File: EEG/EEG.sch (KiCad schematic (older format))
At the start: 1 part

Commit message: ...
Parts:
- gave numbers to parts that had none: 1
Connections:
- net labels added: +5V, GND
- wire segments 0 -> 3
- no-connect marks 0 -> 2
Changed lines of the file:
@@
 $EndDescr
 $Comp
-L Connector:USB_B_Micro J?
+L Connector:USB_B_Micro J1
 U 1 1 603925D3
 P 1950 2800
-F 0 "J?" H 2007 3267 50  0000 C CNN
+F 0 "J1" H 2007 3267 50  0000 C CNN
 F 1 "USB_B_Micro" H 2007 3176 50  0000 C CNN
 F 2 "" H 2100 2750 50  0001 C CNN
@@
 	1    0    0    -1
 $EndComp
+Wire Wire Line
+	1950 3200 1950 3500
+$Comp
+L power:GND #PWR?
+U 1 1 603940FA
+P 1950 3500
+F 0 "#PWR?" H 1950 3250 50  0001 C CNN
+F 1 "GND" H 1955 3327 50  0000 C CNN
+F 2 "" H 1950 3500 50  0001 C CNN
+F 3 "" H 1950 3500 50  0001 C CNN
+	1    1950 3500
+	1    0    0    -1
+$EndComp
+NoConn ~ 1850 3200
+NoConn ~ 2250 3000
+$Comp
+L power:+5V #PWR?
+U 1 1 60394FDA
+P 2500 2300
+F 0 "#PWR?" H 2500 2150 50  0001 C CNN
+F 1 "+5V" H 2515 2473 50  0000 C CNN
+F 2 "" H 2500 2300 50  0001 C CNN
+F 3 "" H 2500 2300 50  0001 C CNN
+	1    2500 2300
+	1    0    0    -1
+$EndComp
+Wire Wire Line
+	2250 2600 2500 2600
+Wire Wire Line
+	2500 2600 2500 2300
 $EndSCHEMATC

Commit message: added stuff to schematic
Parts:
- added C? (x2): 10uF, symbol Device:CP_Small
- added C? (x4): 0.1uF, symbol Device:CP_Small
- added C?: 2.2uF, symbol Device:CP_Small
- added C? (x8): 100nF, symbol Device:CP_Small
- added D? (x3): D_TVS, symbol Device:D_TVS
- added D?: LED, symbol Device:LED
- added D?: D_Schottky_Small, symbol Device:D_Schottky_Small
- added Q? (x2): 2N2219, Package_TO_SOT_THT:TO-39-3, symbol Transistor_BJT:2N2219
- added R? (x3): 2K, symbol Device:R_Small_US
- added R? (x4): 0R, symbol Device:R_Small_US
- added R? (x2): 10K, symbol Device:R_Small_US
- added SW? (x2): SW_Push, symbol Switch:SW_Push
- added U?: AMS1117-3.3, Package_TO_SOT_SMD:SOT-223-3_TabPin2, symbol Regulator_Linear:AMS1117-3.3
- added U?: FT231XS, Package_SO:SSOP-20_3.9x8.7mm_P0.635mm, symbol Interface_USB:FT231XS
- added U?: ESP32-PICO-D4, Package_DFN_QFN:QFN-48-1EP_7x7mm_P0.5mm_EP5.3x5.3mm, symbol RF_Module:ESP32-PICO-D4
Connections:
- net labels added: +3.3V, D+, D-, EN, IO0, RXD, TXD
- net labels removed: +5V
- wire segments 3 -> 145
- no-connect marks 2 -> 10
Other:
- note added: "3.3V power Supply"
- note added: "Push buttons\n"
- note added: "USB to UART\n"
- moved on the sheet: J1

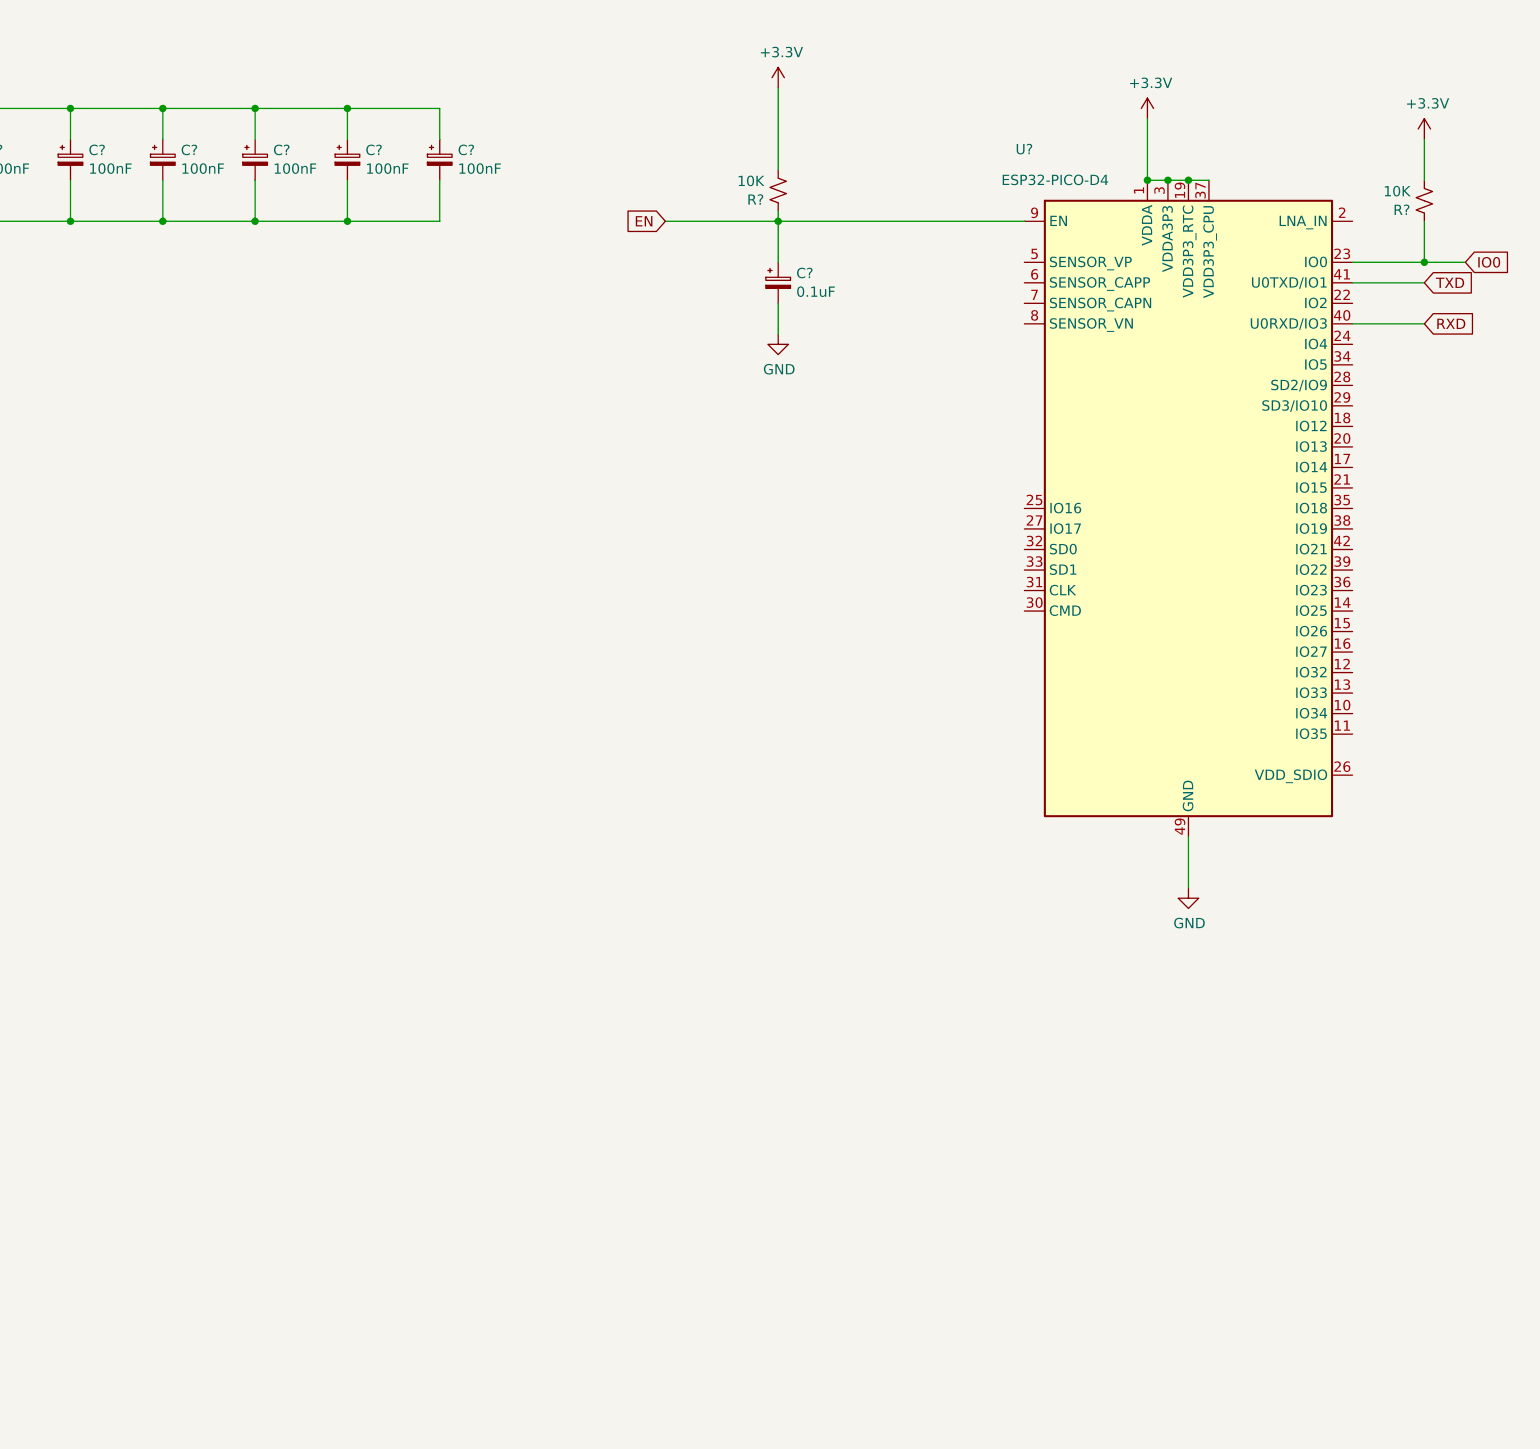
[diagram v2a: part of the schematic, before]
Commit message: ...
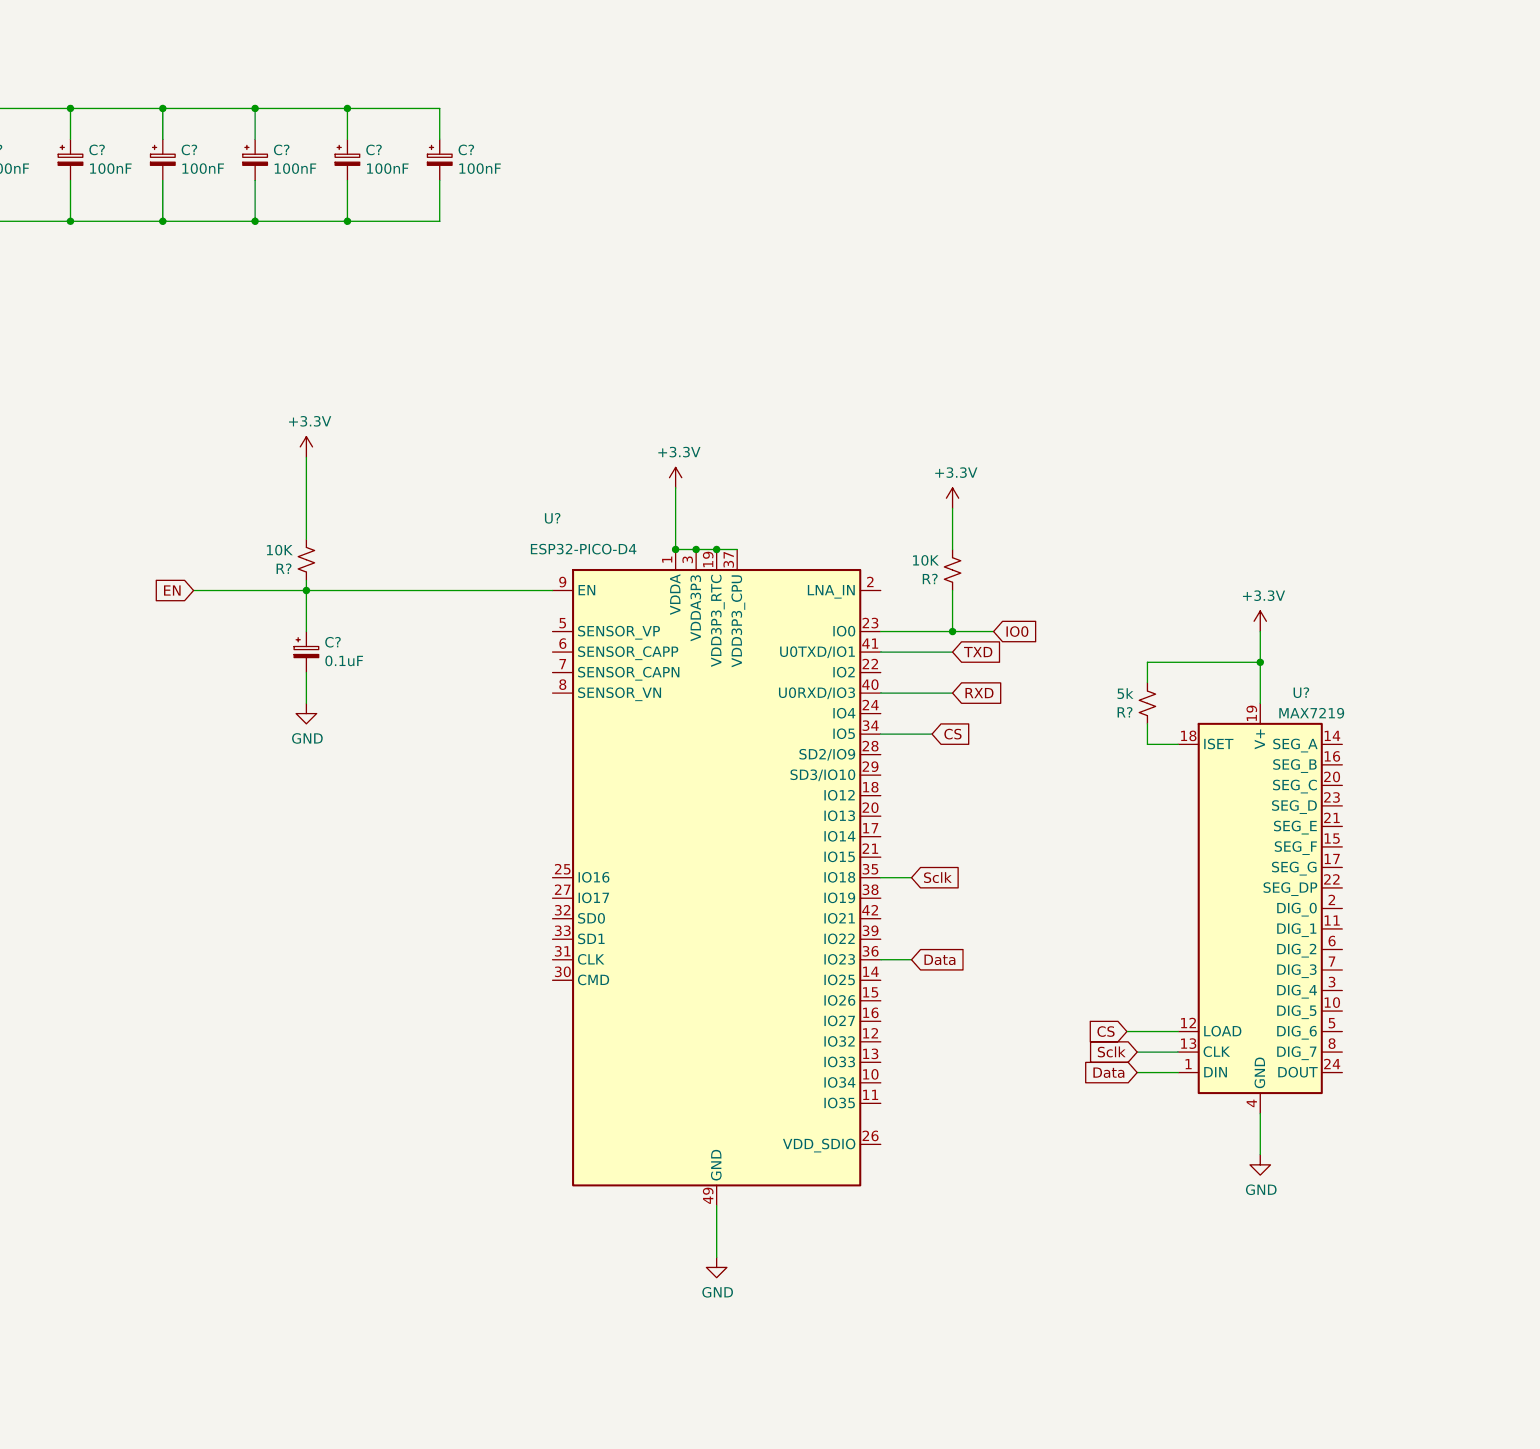
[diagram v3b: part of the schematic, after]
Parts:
- added R?: 5k, symbol Device:R_Small_US
- added U?: MAX7219, symbol Driver_LED:MAX7219
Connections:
- net +3V3: now also R?.2, U?.19 (V+)
- net GND: now also U?.4 (GND), U?.9 (GND)
- net CS: now reaches U?.34 (IO5)
- net CS: now also U?.12 (LOAD)
- net Sclk: now reaches U?.35 (IO18)
- net Sclk: now also U?.13 (CLK)
- net Data: now reaches U?.36 (IO23)
- net Data: now also U?.1 (DIN)
- new net: R?.1, U?.18 (ISET)
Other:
- moved on the sheet: C?, R?, U?
